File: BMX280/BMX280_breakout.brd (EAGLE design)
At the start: 15.2 x 11.2 mm, 2 parts

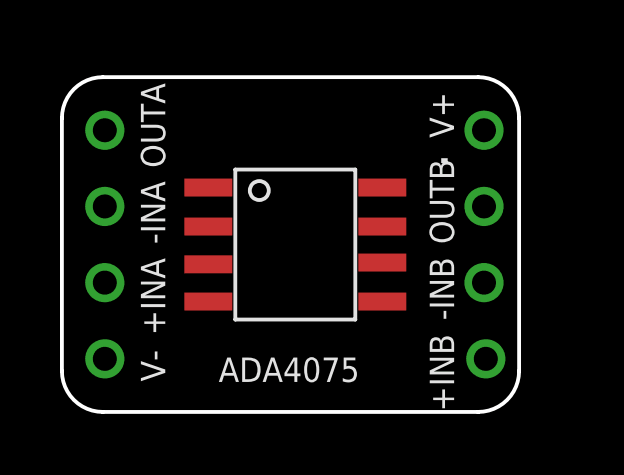
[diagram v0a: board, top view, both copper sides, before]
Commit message: Update new meme.
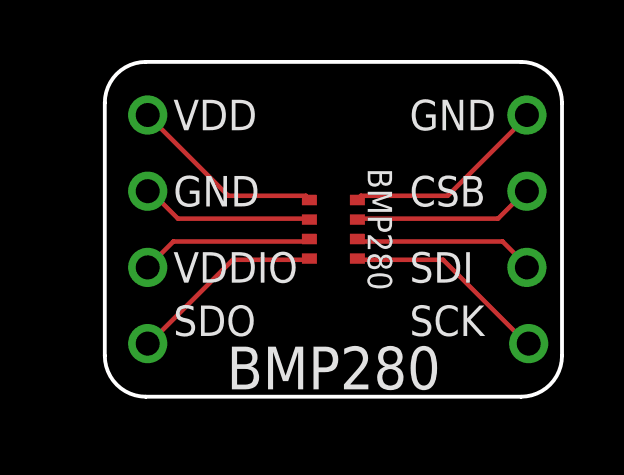
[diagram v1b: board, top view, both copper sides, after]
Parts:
- removed .: ADA4075, FaBo-Opamp:SOIC(NARROW)-8
- removed U$3: 8PIN, FaBo-Breakout:8PIN
- added BMP280: (no value), FaBo-Mems:BOSCH-BMP280
- added U$1: 8PIN, FaBo-Breakout:8PIN
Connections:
- removed net 1: ..1, U$3.1
- removed net 2: ..2, U$3.2
- removed net 3: ..3, U$3.3
- removed net 4: ..4, U$3.4
- removed net 5: ..5, U$3.5
- removed net 6: ..6, U$3.6
- removed net 7: ..7, U$3.7
- removed net 8: ..8, U$3.8
- new net CSB: BMP280.2, U$1.7
- new net GND@1: BMP280.1, U$1.8
- new net GND@7: BMP280.7, U$1.2
- new net SCK: BMP280.4, U$1.5
- new net SDI: BMP280.3, U$1.6
- new net SDO: BMP280.5, U$1.4
- new net VDD: BMP280.8, U$1.1
- new net VDDIO: BMP280.6, U$1.3
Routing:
- net SCK: track 0.00 -> 6.86 mm
- net GND@1: track 0.00 -> 6.86 mm
- net VDD: track 0.00 -> 6.58 mm
- net SDO: track 0.00 -> 6.55 mm
- net SDI: track 0.00 -> 6.06 mm
- net CSB: track 0.00 -> 6.03 mm
- net VDDIO: track 0.00 -> 5.78 mm
- net GND@7: track 0.00 -> 5.77 mm
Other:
- board text added: "BMP280"
- board text added: "CSB"
- board text added: "GND"
- board text added: "SCK"
- board text added: "SDI"
- board text added: "SDO"
- board text added: "VDD"
- board text added: "VDDIO"
- board text removed: "+INA"
- board text removed: "+INB"
- board text removed: "-INA"
- board text removed: "-INB"
- board text removed: "ADA4075"
- board text removed: "OUTA"
- board text removed: "OUTB"
- board text removed: "V+"
- board text removed: "V-"
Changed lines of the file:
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@@
 <setting verticaltext="up"/>
 </settings>
-<grid distance="0.25" unitdist="mm" unit="mm" style="lines" multiple="1" display="yes" altdistance="0.025" altunitdist="inch" altunit="inch"/>
+<grid distance="0.1" unitdist="inch" unit="inch" style="lines" multiple="1" display="no" altdistance="0.025" altunitdist="inch" altunit="inch"/>
 <layers>
 <layer number="1" name="Top" color="4" fill="1" visible="yes" active="yes"/>
@@
 <layer number="49" name="Reference" color="7" fill="1" visible="yes" active="yes"/>
 <layer number="50" name="dxf" color="7" fill="1" visible="no" active="no"/>
-<layer number="51" name="tDocu" color="14" fill="1" visible="yes" active="yes"/>
+<layer number="51" name="tDocu" color="7" fill="1" visible="yes" active="yes"/>
 <layer number="52" name="bDocu" color="7" fill="1" visible="yes" active="yes"/>
 <layer number="53" name="tGND_GNDA" color="7" fill="9" visible="no" active="no"/>
@@
 <layer number="154" name="FabDoc2" color="2" fill="1" visible="no" active="no"/>
 <layer number="155" name="FabDoc3" color="7" fill="15" visible="no" active="no"/>
-<layer number="160" name="O_Dim" color="12" fill="11" visible="yes" active="yes"/>
 <layer number="199" name="Contour" color="7" fill="1" visible="yes" active="yes"/>
-<layer number="200" name="200bmp" color="1" fill="10" visible="yes" active="yes"/>
+<layer number="200" name="200bmp" color="1" fill="10" visible="no" active="yes"/>
 <layer number="201" name="201bmp" color="2" fill="1" visible="no" active="no"/>
 <layer number="202" name="202bmp" color="3" fill="1" visible="no" active="no"/>
@@
 <board>
 <plain>
-<text x="3.794" y="1.262" size="0.8128" layer="21">ADA4075</text>
-<text x="2.016" y="8.398" size="0.8128" layer="21" rot="R90">OUTA</text>
-<text x="2.016" y="5.858" size="0.8128" layer="21" rot="R90">-INA</text>
-<text x="2.016" y="2.818" size="0.8128" layer="21" rot="R90">+INA</text>
-<text x="11.64" y="9.398" size="0.8128" layer="21" rot="R90">V+</text>
-<text x="11.644" y="5.858" size="0.8128" layer="21" rot="R90">OUTB</text>
-<text x="11.644" y="3.318" size="0.8128" layer="21" rot="R90">-INB</text>
-<text x="11.644" y="0.278" size="0.8128" layer="21" rot="R90">+INB</text>
-<text x="2.016" y="1.278" size="0.8128" layer="21" rot="R90">V-</text>
+<text x="4.064" y="1.016" size="1.4224" layer="21">BMP280</text>
+<text x="10.16" y="9.652" size="1.016" layer="21">GND</text>
+<text x="2.286" y="7.112" size="1.016" layer="21">GND</text>
+<text x="2.286" y="9.652" size="1.016" layer="21">VDD</text>
+<text x="10.16" y="7.112" size="1.016" layer="21">CSB</text>
+<text x="10.16" y="4.572" size="1.016" layer="21">SDI</text>
+<text x="10.16" y="2.794" size="1.016" layer="21">SCK</text>
+<text x="2.286" y="4.572" size="1.016" layer="21">VDDIO</text>
+<text x="2.286" y="2.794" size="1.016" layer="21">SDO</text>
 </plain>
 <attributes>
@@
 </class>
 </classes>
-<designrules name="Elecrow_2-layer_eagle_rule">
+<designrules name="SeeedStudio_2layer_DRU_no_angle_20140221">
 <description language="de">&lt;b&gt;EAGLE Design Rules&lt;/b&gt;
 &lt;p&gt;
@@
 necessary adjustments and save your customized
 design rules under a new name.</description>
-<description language="zh">&lt;b&gt;Elecrow EAGLE Design Rules&lt;/b&gt;
+<description language="zh">&lt;b&gt;Seeed Studio EAGLE Design Rules&lt;/b&gt;
 </description>
 <param name="layerSetup" value="(1*16)"/>
-<param name="mtCopper" value="0.035mm 0.035mm 0.035mm 0.035mm 0.035mm 0.035mm 0.035mm 0.035mm 0.035mm 0.035mm 0.035mm 0.035mm 0.035mm 0.035mm 0.035mm 0.035mm"/>
-<param name="mtIsolate" value="1.5mm 0.15mm 0.2mm 0.15mm 0.2mm 0.15mm 0.2mm 0.15mm 0.2mm 0.15mm 0.2mm 0.15mm 0.2mm 0.15mm 0.2mm"/>
+<param name="mtCopper" value="0.035mm 0.0175mm 0.035mm 0.035mm 0.035mm 0.035mm 0.035mm 0.035mm 0.035mm 0.035mm 0.035mm 0.035mm 0.035mm 0.035mm 0.0175mm 0.035mm"/>
+<param name="mtIsolate" value="1.5mm 1.1mm 0.2mm 0.15mm 0.2mm 0.15mm 0.2mm 0.15mm 0.2mm 0.15mm 0.2mm 0.15mm 0.2mm 0.15mm 0.2mm"/>
 <param name="mdWireWire" value="6mil"/>
 <param name="mdWirePad" value="6mil"/>
@@
 </autorouter>
 <elements>
-<element name="U$3" library="FaBo-Breakout" package="8PIN" value="8PIN" x="7.46" y="5.842"/>
-<element name="." library="FaBo-Opamp" package="SOIC(NARROW)-8" value="ADA4075" x="6.35" y="5.842" rot="R270"/>
+<element name="BMP280" library="FaBo-Mems" package="BOSCH-BMP280" value="" x="7.62" y="6.35" rot="R270"/>
+<element name="U$1" library="FaBo-Breakout" package="8PIN" value="8PIN" x="8.89" y="6.35"/>
 </elements>
 <signals>
-<signal name="1">
-<contactref element="U$3" pad="1"/>
-<contactref element="." pad="1"/>
-<wire x1="3.45" y1="7.742" x2="0" y2="9.652" width="0" layer="19" extent="1-1"/>
-</signal>
-<signal name="2">
-<contactref element="U$3" pad="2"/>
-<contactref element="." pad="2"/>
-<wire x1="0" y1="7.112" x2="3.45" y2="6.442" width="0" layer="19" extent="1-1"/>
-</signal>
-<signal name="3">
-<contactref element="U$3" pad="3"/>
-<contactref element="." pad="3"/>
-<wire x1="0" y1="4.572" x2="3.45" y2="5.182" width="0" layer="19" extent="1-1"/>
-</signal>
-<signal name="4">
-<contactref element="U$3" pad="4"/>
-<contactref element="." pad="4"/>
-<wire x1="0" y1="2.032" x2="3.45" y2="3.942" width="0" layer="19" extent="1-1"/>
-</signal>
-<signal name="8">
-<contactref element="U$3" pad="8"/>
-<contactref element="." pad="8"/>
-<wire x1="9.25" y1="7.742" x2="12.64" y2="9.652" width="0" layer="19" extent="1-1"/>
-</signal>
-<signal name="7">
-<contactref element="U$3" pad="7"/>
-<contactref element="." pad="7"/>
-<wire x1="9.25" y1="6.442" x2="12.64" y2="7.112" width="0" layer="19" extent="1-1"/>
-</signal>
-<signal name="6">
-<contactref element="U$3" pad="6"/>
-<contactref element="." pad="6"/>
-<wire x1="9.25" y1="5.242" x2="12.64" y2="4.572" width="0" layer="19" extent="1-1"/>
-</signal>
-<signal name="5">
-<contactref element="U$3" pad="5"/>
-<contactref element="." pad="5"/>
-<wire x1="12.7" y1="2.032" x2="9.25" y2="3.942" width="0" layer="19" extent="1-1"/>
+<signal name="CSB">
+<contactref element="U$1" pad="7"/>
+<contactref element="BMP280" pad="2"/>
+<wire x1="13.1064" y1="6.7056" x2="8.5344" y2="6.7056" width="0.1524" layer="1"/>
+<wire x1="14.0208" y1="7.62" x2="13.1064" y2="6.7056" width="0.1524" layer="1"/>
+<wire x1="8.5344" y1="6.7056" x2="8.42" y2="6.675" width="0.1524" layer="1"/>
+<wire x1="14.0208" y1="7.62" x2="14.07" y2="7.62" width="0.1524" layer="1"/>
+</signal>
+<signal name="SDI">
+<contactref element="BMP280" pad="3"/>
+<contactref element="U$1" pad="6"/>
+<wire x1="13.2588" y1="5.9436" x2="8.5344" y2="5.9436" width="0.1524" layer="1"/>
+<wire x1="14.0208" y1="5.1816" x2="13.2588" y2="5.9436" width="0.1524" layer="1"/>
+<wire x1="8.5344" y1="5.9436" x2="8.42" y2="6.025" width="0.1524" layer="1"/>
+<wire x1="14.0208" y1="5.1816" x2="14.07" y2="5.08" width="0.1524" layer="1"/>
+</signal>
+<signal name="SCK">
+<contactref element="BMP280" pad="4"/>
+<contactref element="U$1" pad="5"/>
+<wire x1="11.2776" y1="5.334" x2="8.5344" y2="5.334" width="0.1524" layer="1"/>
+<wire x1="14.0208" y1="2.5908" x2="11.2776" y2="5.334" width="0.1524" layer="1"/>
+<wire x1="8.5344" y1="5.334" x2="8.42" y2="5.375" width="0.1524" layer="1"/>
+<wire x1="14.0208" y1="2.5908" x2="14.13" y2="2.54" width="0.1524" layer="1"/>
+</signal>
+<signal name="GND@1">
+<contactref element="BMP280" pad="1"/>
+<contactref element="U$1" pad="8"/>
+<wire x1="11.43" y1="7.4676" x2="8.5344" y2="7.4676" width="0.1524" layer="1"/>
+<wire x1="14.0208" y1="10.0584" x2="11.43" y2="7.4676" width="0.1524" layer="1"/>
+<wire x1="8.5344" y1="7.4676" x2="8.42" y2="7.325" width="0.1524" layer="1"/>
+<wire x1="14.0208" y1="10.0584" x2="14.07" y2="10.16" width="0.1524" layer="1"/>
+</signal>
+<signal name="VDD">
+<contactref element="BMP280" pad="8"/>
+<contactref element="U$1" pad="1"/>
+<wire x1="4.1148" y1="7.4676" x2="6.7056" y2="7.4676" width="0.1524" layer="1"/>
+<wire x1="1.524" y1="10.0584" x2="4.1148" y2="7.4676" width="0.1524" layer="1"/>
+<wire x1="6.7056" y1="7.4676" x2="6.82" y2="7.325" width="0.1524" layer="1"/>
+<wire x1="1.524" y1="10.0584" x2="1.43" y2="10.16" width="0.1524" layer="1"/>
+</signal>
+<signal name="GND@7">
+<contactref element="BMP280" pad="7"/>
+<contactref element="U$1" pad="2"/>
+<wire x1="2.4384" y1="6.7056" x2="6.7056" y2="6.7056" width="0.1524" layer="1"/>
+<wire x1="1.524" y1="7.62" x2="2.4384" y2="6.7056" width="0.1524" layer="1"/>
+<wire x1="6.7056" y1="6.7056" x2="6.82" y2="6.675" width="0.1524" layer="1"/>
+<wire x1="1.524" y1="7.62" x2="1.43" y2="7.62" width="0.1524" layer="1"/>
+</signal>
+<signal name="VDDIO">
+<contactref element="BMP280" pad="6"/>
+<contactref element="U$1" pad="3"/>
+<wire x1="2.286" y1="5.9436" x2="6.7056" y2="5.9436" width="0.1524" layer="1"/>
+<wire x1="1.524" y1="5.1816" x2="2.286" y2="5.9436" width="0.1524" layer="1"/>
+<wire x1="6.7056" y1="5.9436" x2="6.82" y2="6.025" width="0.1524" layer="1"/>
+<wire x1="1.524" y1="5.1816" x2="1.43" y2="5.08" width="0.1524" layer="1"/>
+</signal>
+<signal name="SDO">
+<contactref element="BMP280" pad="5"/>
+<contactref element="U$1" pad="4"/>
+<wire x1="4.2672" y1="5.334" x2="6.7056" y2="5.334" width="0.1524" layer="1"/>
+<wire x1="1.524" y1="2.5908" x2="4.2672" y2="5.334" width="0.1524" layer="1"/>
+<wire x1="6.7056" y1="5.334" x2="6.82" y2="5.375" width="0.1524" layer="1"/>
+<wire x1="1.524" y1="2.5908" x2="1.43" y2="2.54" width="0.1524" layer="1"/>
 </signal>
 </signals>
-<errors>
-</errors>
 </board>
 </drawing>
